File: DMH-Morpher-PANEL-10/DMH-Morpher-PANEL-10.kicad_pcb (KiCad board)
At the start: 2 copper layers, 100 x 200 mm, 29 parts, among them J0 Panel_GND_Solder_Wire_Pad

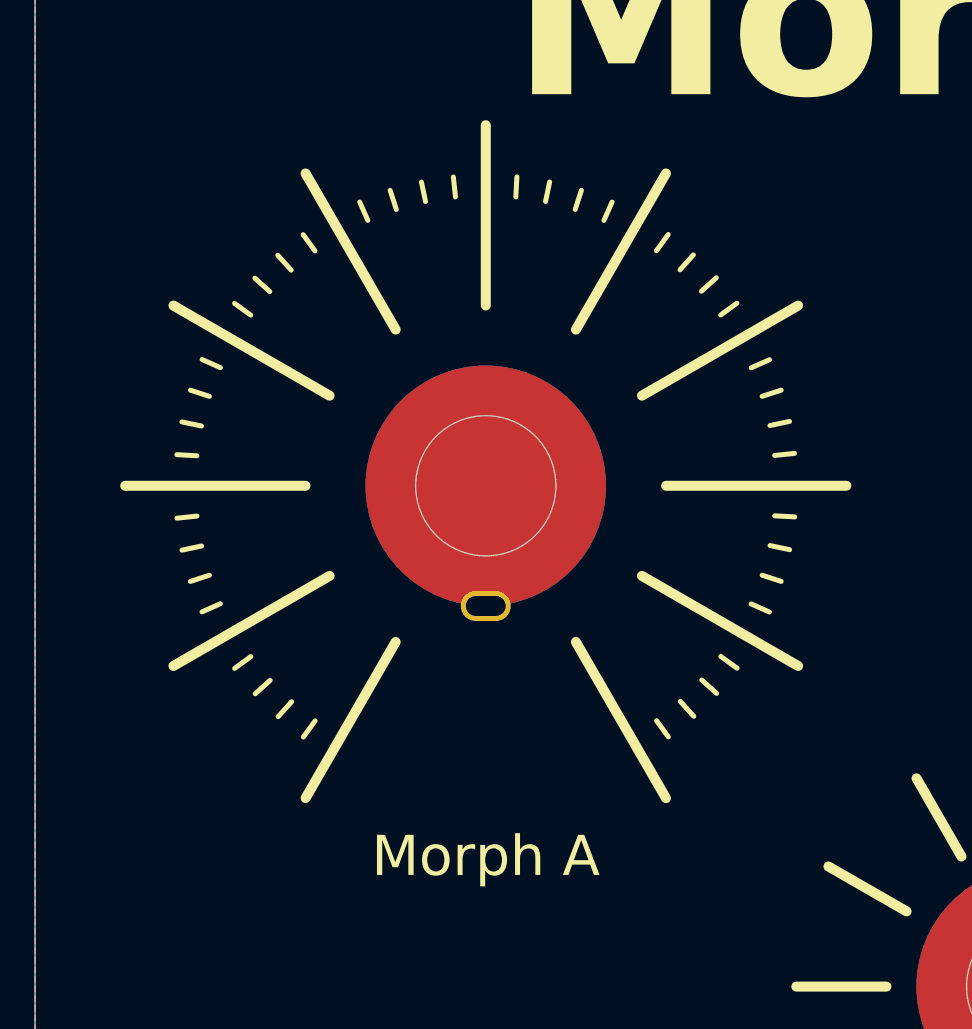
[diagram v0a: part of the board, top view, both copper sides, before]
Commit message: Front panel art ongoing
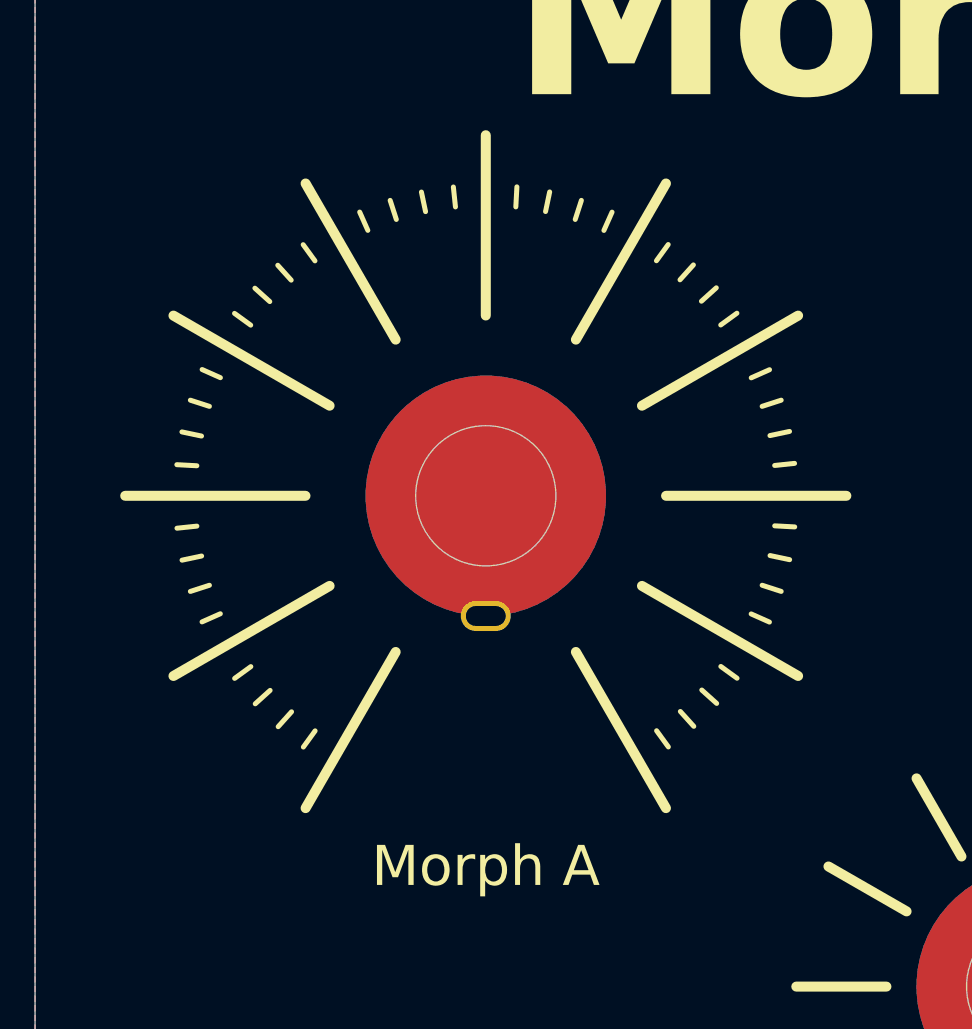
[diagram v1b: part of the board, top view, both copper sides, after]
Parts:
- moved H7 0.50 mm to (72.5, 60.5)
